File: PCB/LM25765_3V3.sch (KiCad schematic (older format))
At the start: 8 parts

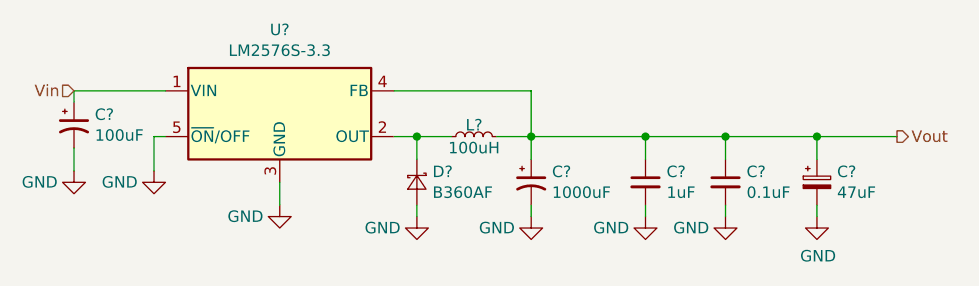
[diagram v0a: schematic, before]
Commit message: Cleanup
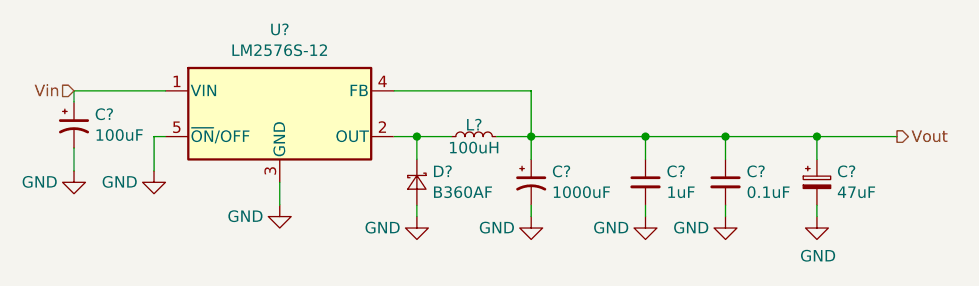
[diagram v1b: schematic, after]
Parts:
- U?: value LM2576S-3.3 -> LM2576S-12
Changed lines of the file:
@@
 AR Path="/5E880E11/5E9C913B/5B713F8D" Ref="U?"  Part="1"
 F 0 "U?" H 5200 4117 50  0000 C CNN
-F 1 "LM2576S-3.3" H 5200 4026 50  0000 C CNN
+F 1 "LM2576S-12" H 5200 4026 50  0000 C CNN
 F 2 "Package_TO_SOT_SMD:TO-263-5_TabPin3" H 5200 3500 50  0001 L CIN
 F 3 "http://www.ti.com/lit/ds/symlink/lm2576.pdf" H 5200 3750 50  0001 C CNN
